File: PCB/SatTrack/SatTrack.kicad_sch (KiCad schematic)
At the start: 10 parts

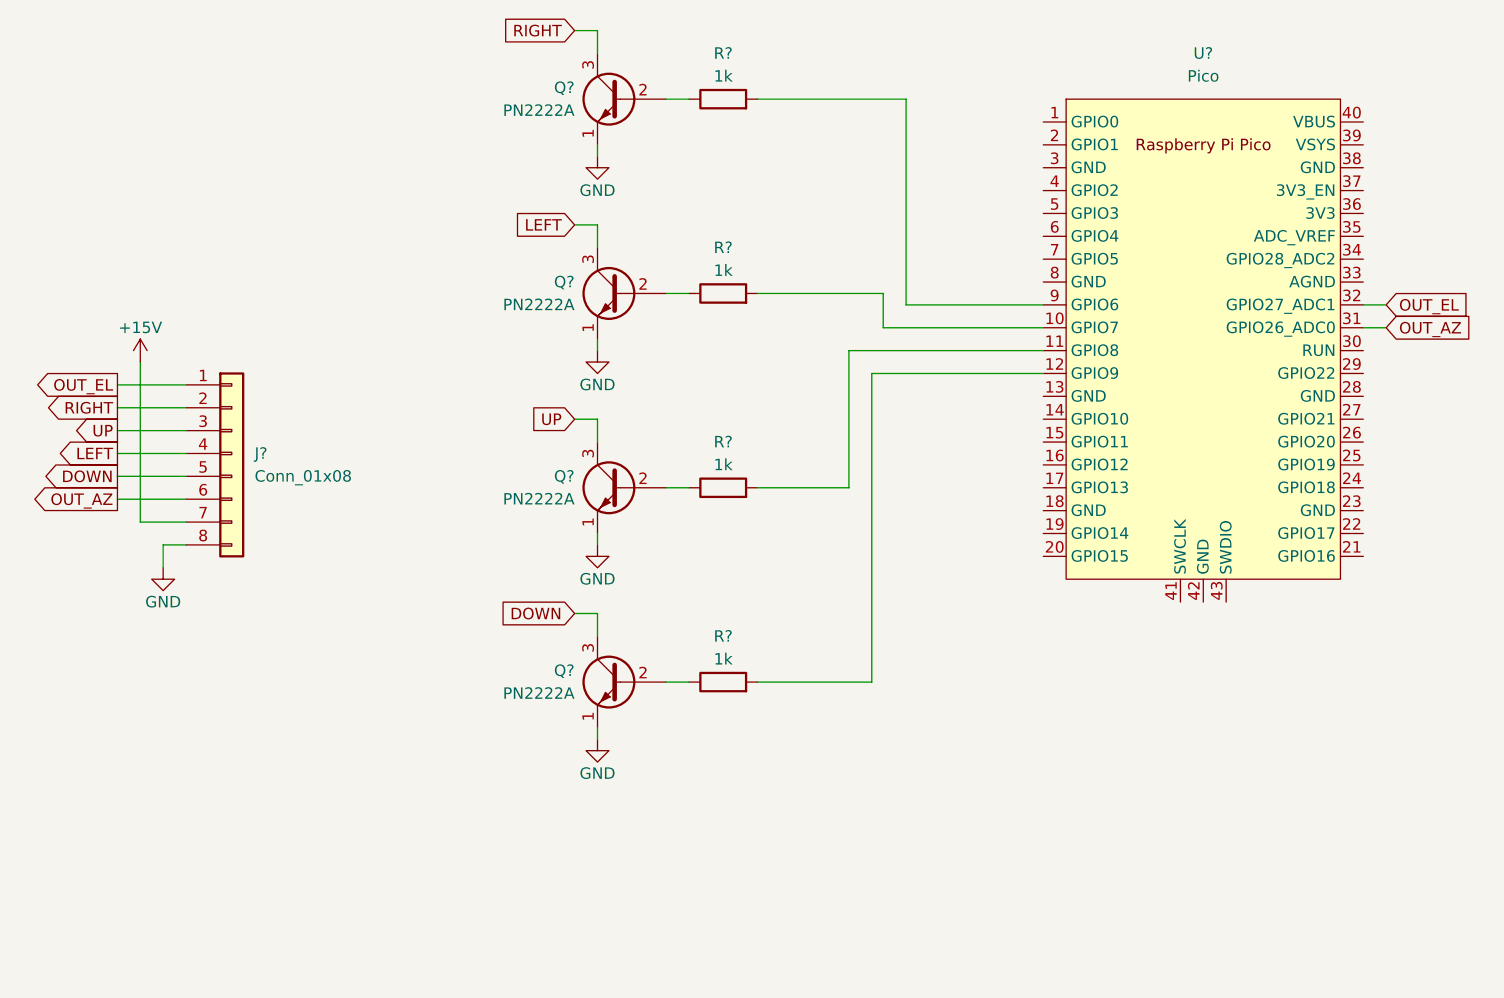
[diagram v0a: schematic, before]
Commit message: add Documentation
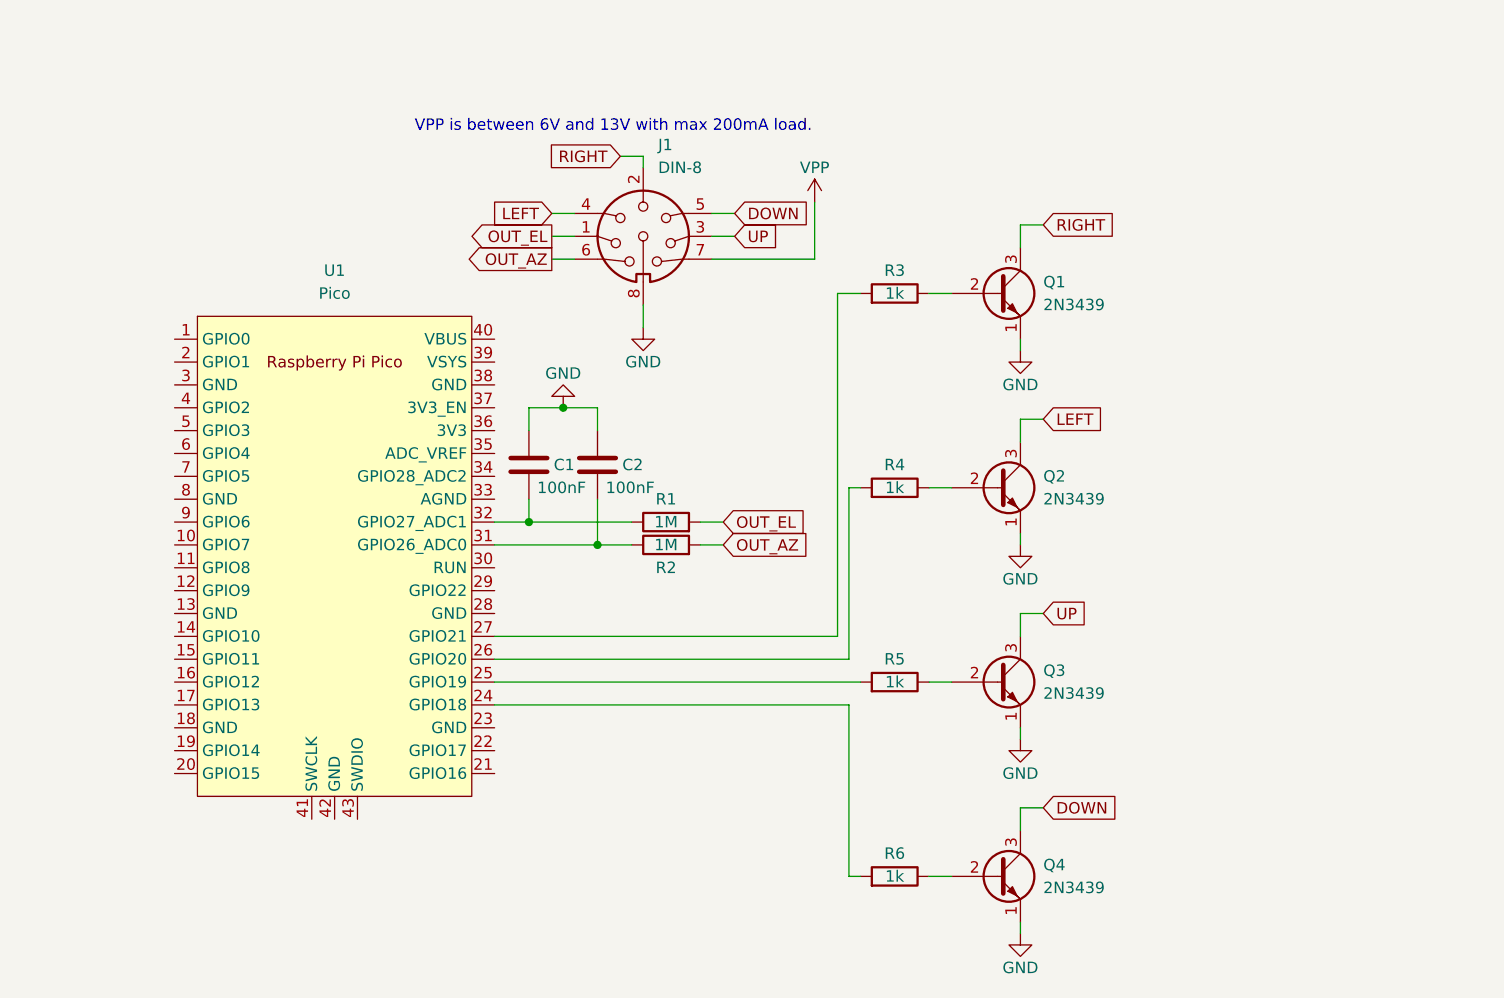
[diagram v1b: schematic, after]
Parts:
- removed J?: Conn_01x08, symbol Connector_Generic:Conn_01x08
- removed Q? (x4): PN2222A, Package_TO_SOT_THT:TO-92_Inline, symbol Transistor_BJT:PN2222A
- removed R? (x4): 1k, symbol Device:R
- added C1, C2: 100nF, symbol Device:C
- added J1: DIN-8, symbol Connector:DIN-8
- added Q1, Q2, Q3, Q4: 2N3439, Package_TO_SOT_THT:TO-92_Inline, symbol Transistor_BJT:PN2222A
- added R1, R2: 1M, symbol Device:R
- added R3, R4, R5, R6: 1k, symbol Device:R
- gave numbers to parts that had none: 1
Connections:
- net DOWN: now also J1.5, Q4.3 (C)
- net GND: now also C1.2, C2.2, J1.8, Q1.1 (E), Q2.1 (E), Q3.1 (E), Q4.1 (E)
- net LEFT: now also J1.4, Q2.3 (C)
- net OUT_AZ: now also J1.6, R2.2; no longer U1.31 (GPIO26_ADC0)
- net OUT_EL: now also J1.1, R1.2; no longer U1.32 (GPIO27_ADC1)
- net RIGHT: now also J1.2, Q1.3 (C)
- net UP: now also J1.3, Q3.3 (C)
- net at U1.24 (GPIO18): now also R6.2
- net at U1.25 (GPIO19): now also R5.2
- net at U1.26 (GPIO20): now also R4.2
- net at U1.27 (GPIO21): now also R3.2
- new net: Q3.2 (B), R5.1
- new net: Q1.2 (B), R3.1
- new net: C1.1, R1.1, U1.32 (GPIO27_ADC1)
- new net: C2.1, R2.1, U1.31 (GPIO26_ADC0)
- new net: Q4.2 (B), R6.1
- new net: Q2.2 (B), R4.1
- new net VPP: J1.7
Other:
- note added: "VPP is between 6V and 13V with max 200mA load."
- moved on the sheet: U1
